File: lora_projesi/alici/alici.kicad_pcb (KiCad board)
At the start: 4 copper layers, 88 x 102 mm, 127 parts, among them J1 USB-C, J2 SMA, J3 RJ45, J4 u.FL (ANA ANTEN), J5 12 V GIRIS, J6 LAMBA, J7 MICRO-SIM, J8 u.FL (YARDIMCI ANTEN, ISTEGE 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, K1 SRD-12VDC-SL-A, Q1 AO3401A, Q2 MMBT2222A, Q3 MMBT2222A, Q4 MMBT2222A, SW1 DUGME, U1 ESP32-S3-WROOM-1-N4, U10 SIM7600SA, U11 AP2112K-3.3, U12 ESDA6V1-5SC6, U4 RFM95W-915S2, U5 TPS62933DRLR, U6 TPS62933DRLR, U7 USBLC6-2SC6, U8 TXB0104PW, U9 W5500, Y1 25 MHz

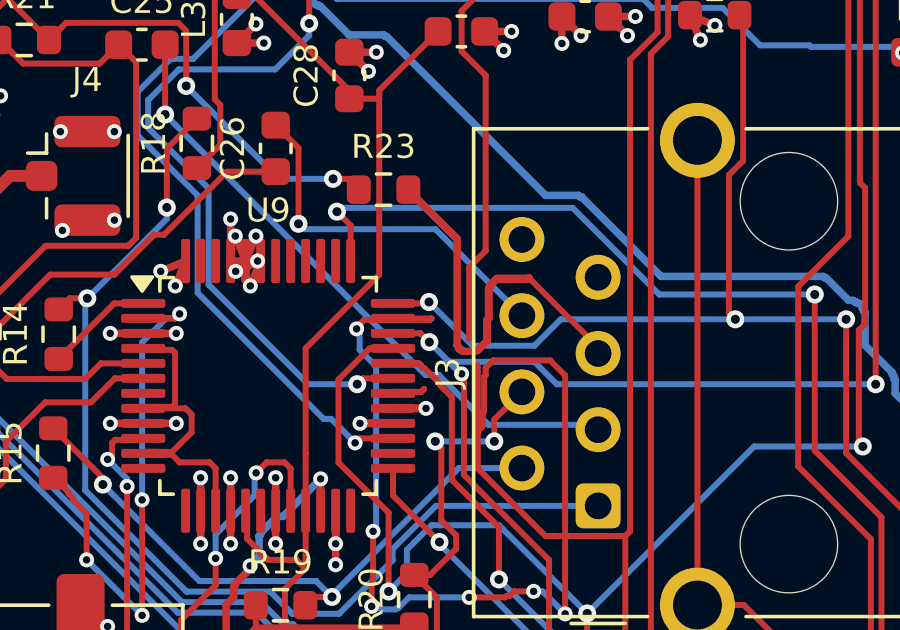
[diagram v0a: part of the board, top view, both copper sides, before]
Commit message: izgara: adim adim surec dongusu
Co-Authored-By: Claude Sonnet 5.5 <noreply@anthropic.com>
Claude-Session: https://claude.ai/code/session_01Q71gHQtKJ86ZE2CtYTYSwP
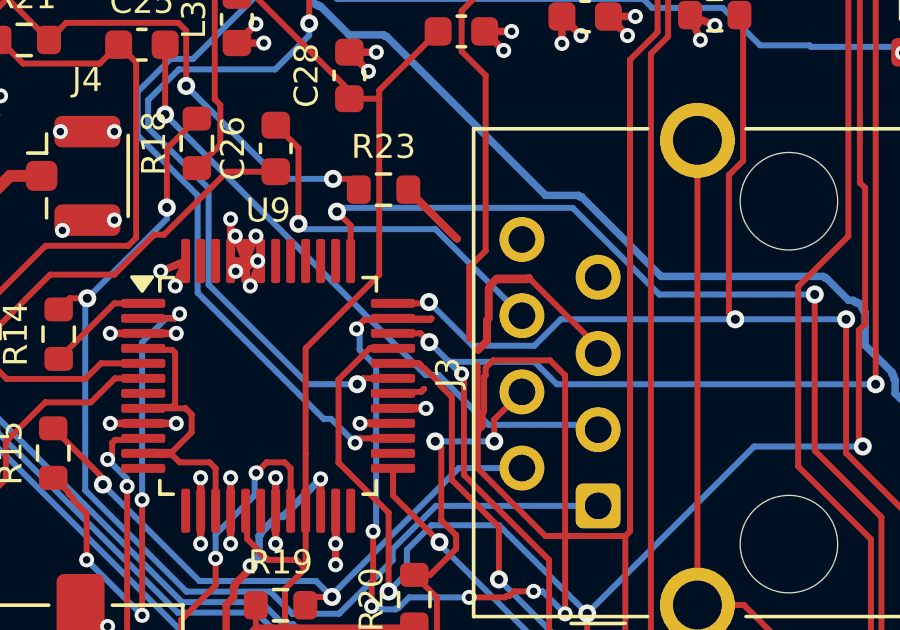
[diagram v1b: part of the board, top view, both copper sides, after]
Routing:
- net RCT: track 21.1 -> 16.7 mm
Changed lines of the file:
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@@
   (segment (start 76.3781 89.9365) (end 76.3781 87.7731) (width 0.2) (layer "F.Cu") (net 19))
   (segment (start 76.325 87.72) (end 77.15 86.895) (width 0.2) (layer "F.Cu") (net 19))
-  (segment (start 61.75 61.95) (end 61.2 61.4) (width 0.2) (layer "F.Cu") (net 20))
-  (segment (start 61.2 61.4) (end 61.15 61.4) (width 0.2) (layer "F.Cu") (net 20))
+  (segment (start 61.75 61.95) (end 61.75 62) (width 0.2) (layer "F.Cu") (net 20))
   (segment (start 61.15 61.4) (end 61.05 61.3) (width 0.2) (layer "F.Cu") (net 20))
   (segment (start 61 61.25) (end 61.05 61.3) (width 0.2) (layer "F.Cu") (net 20))
@@
   (segment (start 60.1625 61.25) (end 61.0447 61.25) (width 0.2) (layer "F.Cu") (net 20))
   (segment (start 62.1241 62.3294) (end 62.1241 65.1352) (width 0.2) (layer "F.Cu") (net 20))
-  (segment (start 61.75 62) (end 61.75 61.95) (width 0.2) (layer "F.Cu") (net 20))
+  (segment (start 61.2 61.4) (end 61.75 61.95) (width 0.2) (layer "F.Cu") (net 20))
+  (segment (start 61.15 61.4) (end 61.2 61.4) (width 0.2) (layer "F.Cu") (net 20))
   (segment (start 61.05 61.3) (end 61.1 61.3) (width 0.2) (layer "F.Cu") (net 20))
   (segment (start 62.1241 65.1352) (end 63.6935 66.7046) (width 0.2) (layer "F.Cu") (net 20))
@@
   (segment (start 63.35 59.75) (end 63.35 58.75) (width 0.25) (layer "F.Cu") (net 56))
   (segment (start 67 60.7082) (end 64.6818 58.39) (width 0.2) (layer "F.Cu") (net 56))
-  (segment (start 62.3 60.65) (end 62.35 60.7) (width 0.25) (layer "F.Cu") (net 56))
   (segment (start 63.35 58.75) (end 63.4 58.7) (width 0.25) (layer "F.Cu") (net 56))
-  (segment (start 62.9 60.85) (end 62.95 60.8) (width 0.25) (layer "F.Cu") (net 56))
-  (segment (start 62.45 60.8) (end 62.5 60.85) (width 0.25) (layer "F.Cu") (net 56))
   (segment (start 63.6 58.45) (end 64.65 58.45) (width 0.25) (layer "F.Cu") (net 56))
   (segment (start 63.4 58.65) (end 63.6 58.45) (width 0.25) (layer "F.Cu") (net 56))
@@
   (segment (start 63 60.8) (end 63.3 60.5) (width 0.25) (layer "F.Cu") (net 56))
   (segment (start 63.6 58.45) (end 64.65 58.45) (width 0.25) (layer "F.Cu") (net 56))
-  (segment (start 62.35 60.75) (end 62.4 60.8) (width 0.25) (layer "F.Cu") (net 56))
-  (segment (start 62.95 60.8) (end 63 60.8) (width 0.25) (layer "F.Cu") (net 56))
   (segment (start 63.3 59.8) (end 63.35 59.75) (width 0.25) (layer "F.Cu") (net 56))
   (segment (start 63.35 59.75) (end 63.35 58.75) (width 0.25) (layer "F.Cu") (net 56))
@@
   (segment (start 63.3 60.5) (end 63.3 59.8) (width 0.25) (layer "F.Cu") (net 56))
   (segment (start 64.65 58.45) (end 64.7 58.4) (width 0.25) (layer "F.Cu") (net 56))
-  (segment (start 62.5 60.85) (end 62.9 60.85) (width 0.25) (layer "F.Cu") (net 56))
-  (segment (start 62.4 60.8) (end 62.45 60.8) (width 0.25) (layer "F.Cu") (net 56))
   (segment (start 63 60.8) (end 63.3 60.5) (width 0.25) (layer "F.Cu") (net 56))
-  (segment (start 62.3 57.1) (end 62.3 60.65) (width 0.25) (layer "F.Cu") (net 56))
-  (segment (start 62.35 60.7) (end 62.35 60.75) (width 0.25) (layer "F.Cu") (net 56))
   (segment (start 64.6818 58.39) (end 63.6025 58.39) (width 0.2) (layer "F.Cu") (net 56))
   (segment (start 63.3 60.5) (end 63.3 59.8) (width 0.25) (layer "F.Cu") (net 56))
@@
   (segment (start 61.1 62.2) (end 61.2 62.1) (width 0.2) (layer "F.Cu") (net 91))
   (segment (start 62.2888 42.2045) (end 62.4655 42.0278) (width 0.2) (layer "F.Cu") (net 91))
+  (segment (start 61.1 62.2) (end 61.2 62.1) (width 0.2) (layer "F.Cu") (net 91))
   (segment (start 63.25 48.7) (end 63.25 46.85) (width 0.2) (layer "F.Cu") (net 91))
   (segment (start 62.2888 45.1841) (end 62.2888 42.2045) (width 0.2) (layer "F.Cu") (net 91))
